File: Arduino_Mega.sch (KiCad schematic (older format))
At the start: 0 parts

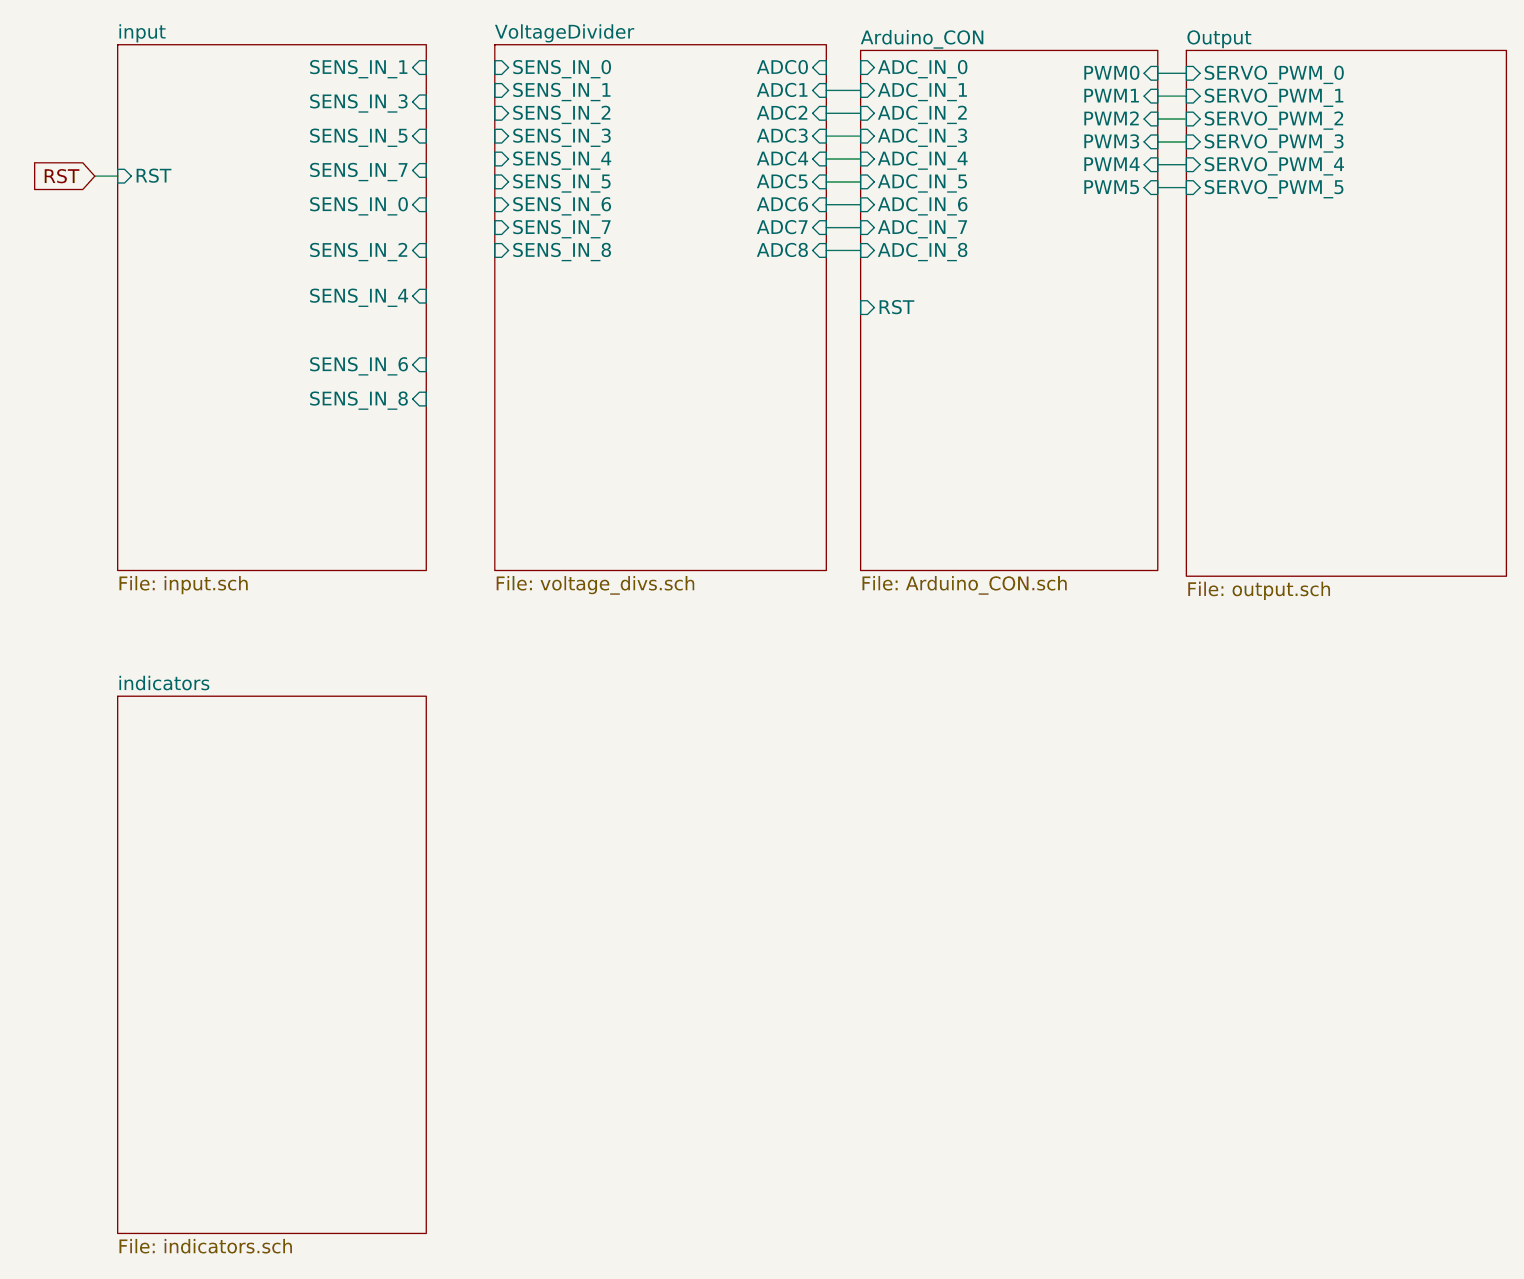
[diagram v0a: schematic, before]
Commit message: Netlist and PCB generated
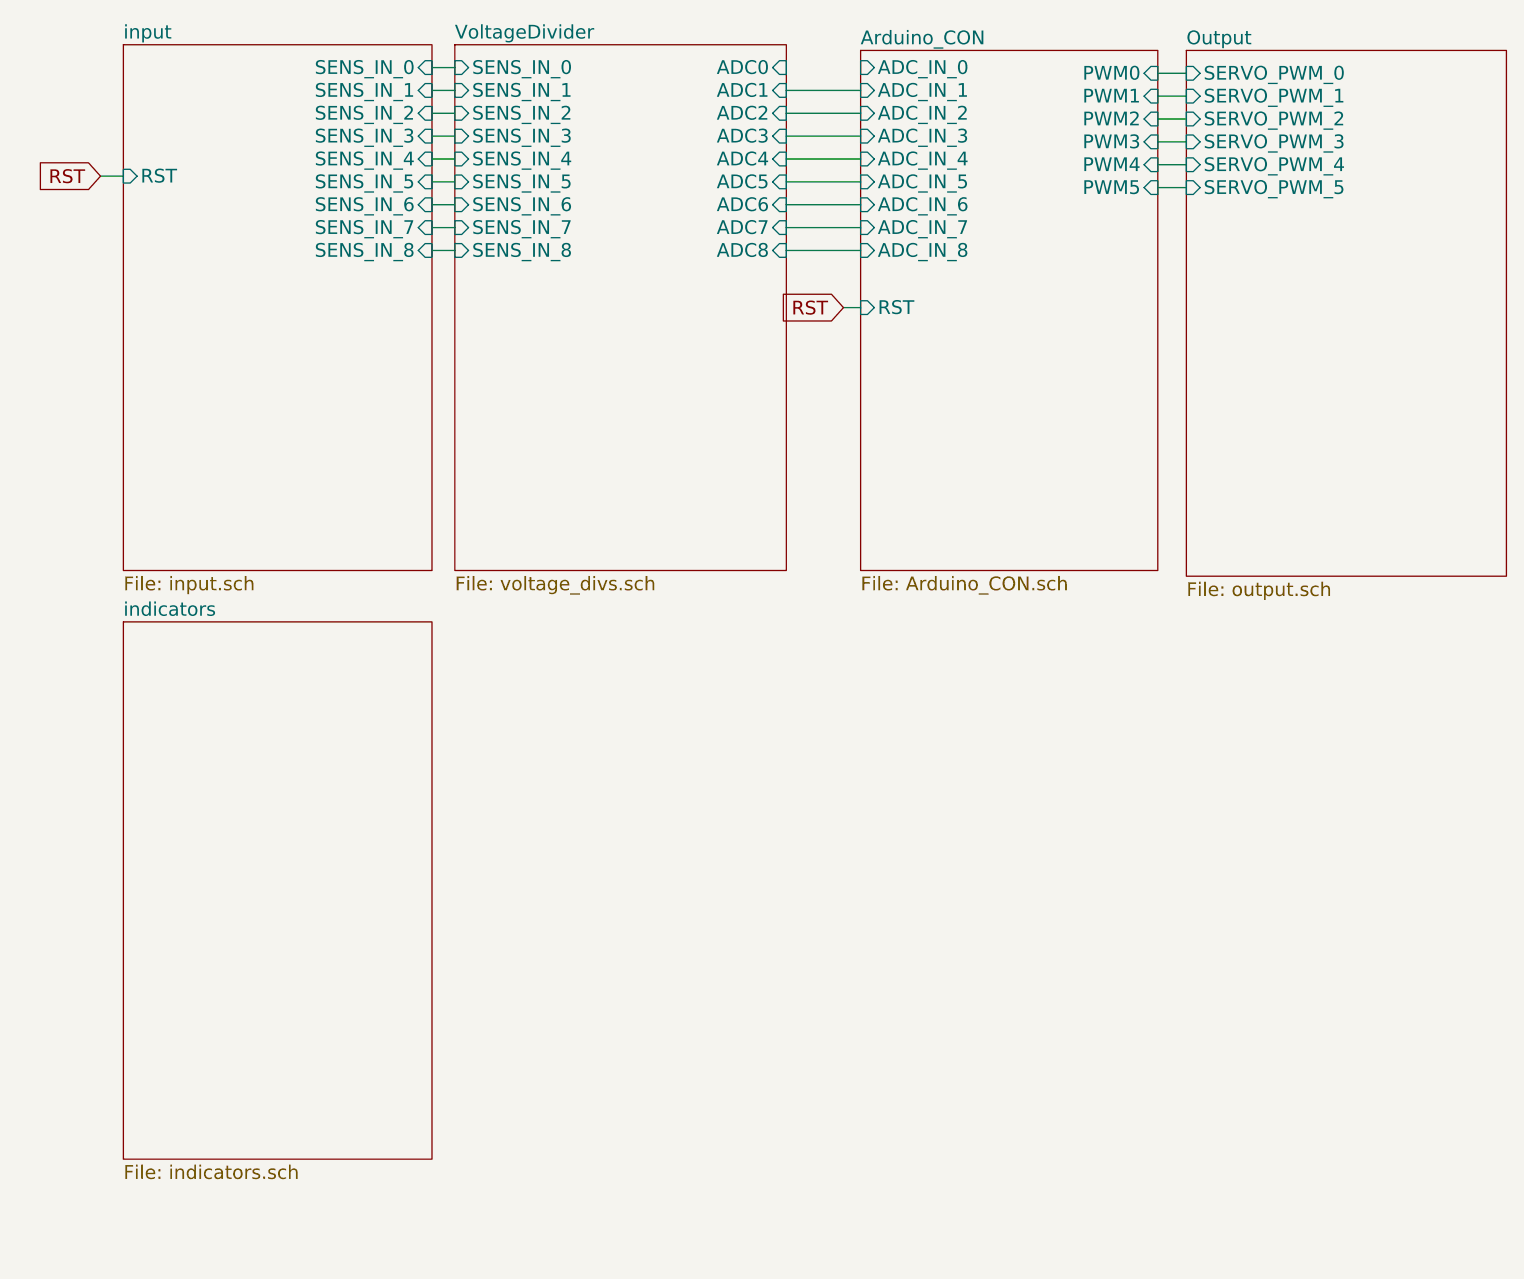
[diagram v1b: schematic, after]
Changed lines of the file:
@@
 $EndDescr
 $Sheet
-S 3100 800  1450 2300
+S 2925 800  1450 2300
 U 57FD64B2
 F0 "VoltageDivider" 60
 F1 "voltage_divs.sch" 60
-F2 "ADC0" I R 4550 900 60
-F3 "SENS_IN_0" I L 3100 900 60
-F4 "ADC1" I R 4550 1000 60
-F5 "SENS_IN_1" I L 3100 1000 60
-F6 "ADC2" I R 4550 1100 60
-F7 "SENS_IN_2" I L 3100 1100 60
-F8 "ADC3" I R 4550 1200 60
-F9 "SENS_IN_3" I L 3100 1200 60
-F10 "ADC4" I R 4550 1300 60
-F11 "SENS_IN_4" I L 3100 1300 60
-F12 "ADC5" I R 4550 1400 60
-F13 "SENS_IN_5" I L 3100 1400 60
-F14 "ADC6" I R 4550 1500 60
-F15 "SENS_IN_6" I L 3100 1500 60
-F16 "ADC7" I R 4550 1600 60
-F17 "SENS_IN_7" I L 3100 1600 60
-F18 "ADC8" I R 4550 1700 60
-F19 "SENS_IN_8" I L 3100 1700 60
+F2 "ADC0" I R 4375 900 60
+F3 "SENS_IN_0" I L 2925 900 60
+F4 "ADC1" I R 4375 1000 60
+F5 "SENS_IN_1" I L 2925 1000 60
+F6 "ADC2" I R 4375 1100 60
+F7 "SENS_IN_2" I L 2925 1100 60
+F8 "ADC3" I R 4375 1200 60
+F9 "SENS_IN_3" I L 2925 1200 60
+F10 "ADC4" I R 4375 1300 60
+F11 "SENS_IN_4" I L 2925 1300 60
+F12 "ADC5" I R 4375 1400 60
+F13 "SENS_IN_5" I L 2925 1400 60
+F14 "ADC6" I R 4375 1500 60
+F15 "SENS_IN_6" I L 2925 1500 60
+F16 "ADC7" I R 4375 1600 60
+F17 "SENS_IN_7" I L 2925 1600 60
+F18 "ADC8" I R 4375 1700 60
+F19 "SENS_IN_8" I L 2925 1700 60
 $EndSheet
 $Sheet
@@
 $EndSheet
 $Sheet
-S 1450 800  1350 2300
+S 1475 800  1350 2300
 U 57FDD173
 F0 "input" 60
 F1 "input.sch" 60
-F2 "SENS_IN_1" I R 2800 900 60
-F3 "SENS_IN_3" I R 2800 1050 60
-F4 "SENS_IN_5" I R 2800 1200 60
-F5 "SENS_IN_7" I R 2800 1350 60
-F6 "SENS_IN_0" I R 2800 1500 60
-F7 "SENS_IN_2" I R 2800 1700 60
-F8 "SENS_IN_4" I R 2800 1900 60
-F9 "SENS_IN_6" I R 2800 2200 60
-F10 "SENS_IN_8" I R 2800 2350 60
-F11 "RST" I L 1450 1375 60
+F2 "RST" I L 1475 1375 60
+F3 "SENS_IN_1" I R 2825 1000 60
+F4 "SENS_IN_3" I R 2825 1200 60
+F5 "SENS_IN_5" I R 2825 1400 60
+F6 "SENS_IN_7" I R 2825 1600 60
+F7 "SENS_IN_0" I R 2825 900 60
+F8 "SENS_IN_2" I R 2825 1100 60
+F9 "SENS_IN_4" I R 2825 1300 60
+F10 "SENS_IN_6" I R 2825 1500 60
+F11 "SENS_IN_8" I R 2825 1700 60
 $EndSheet
 $Sheet
-S 1450 3650 1350 2350
+S 1475 3325 1350 2350
 U 57FDEC0D
 F0 "indicators" 60
 F1 "indicators.sch" 60
 $EndSheet
-Text GLabel 1350 1375 0    60   Input ~ 0
+Text GLabel 1375 1375 0    60   Input ~ 0
 RST
 $Sheet
@@
 $EndSheet
 Wire Wire Line
-	1350 1375 1450 1375
+	1375 1375 1475 1375
 Wire Wire Line
-	4550 1000 4700 1000
+	4375 1000 4700 1000
 Wire Wire Line
-	4550 1100 4700 1100
+	4375 1100 4700 1100
 Wire Wire Line
-	4550 1200 4700 1200
+	4375 1200 4700 1200
 Wire Wire Line
-	4550 1300 4700 1300
+	4375 1300 4700 1300
 Wire Wire Line
-	4550 1400 4700 1400
+	4375 1400 4700 1400
 Wire Wire Line
-	4700 1500 4550 1500
+	4700 1500 4375 1500
 Wire Wire Line
-	4550 1600 4700 1600
+	4375 1600 4700 1600
 Wire Wire Line
-	4700 1700 4550 1700
+	4700 1700 4375 1700
 Wire Wire Line
 	6000 925  6125 925
@@
 Wire Wire Line
 	6125 1425 6000 1425
+Wire Wire Line
+	2925 900  2825 900
+Wire Wire Line
+	2825 1000 2925 1000
+Wire Wire Line
+	2925 1100 2825 1100
+Wire Wire Line
+	2825 1200 2925 1200
+Wire Wire Line
+	2925 1300 2825 1300
+Wire Wire Line
+	2825 1400 2925 1400
+Wire Wire Line
+	2825 1500 2925 1500
+Wire Wire Line
+	2925 1600 2825 1600
+Wire Wire Line
+	2825 1700 2925 1700
+Text GLabel 4625 1950 0    60   Input ~ 0
+RST
+Wire Wire Line
+	4625 1950 4700 1950
 $EndSCHEMATC
